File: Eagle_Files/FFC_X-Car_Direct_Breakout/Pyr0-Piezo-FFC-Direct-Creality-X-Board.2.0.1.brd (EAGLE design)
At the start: 48.1 x 50.7 mm, 11 parts, among them J1 FFC_MOLEX_0.5MM, J2 FFC_MOLEX_0.5MM

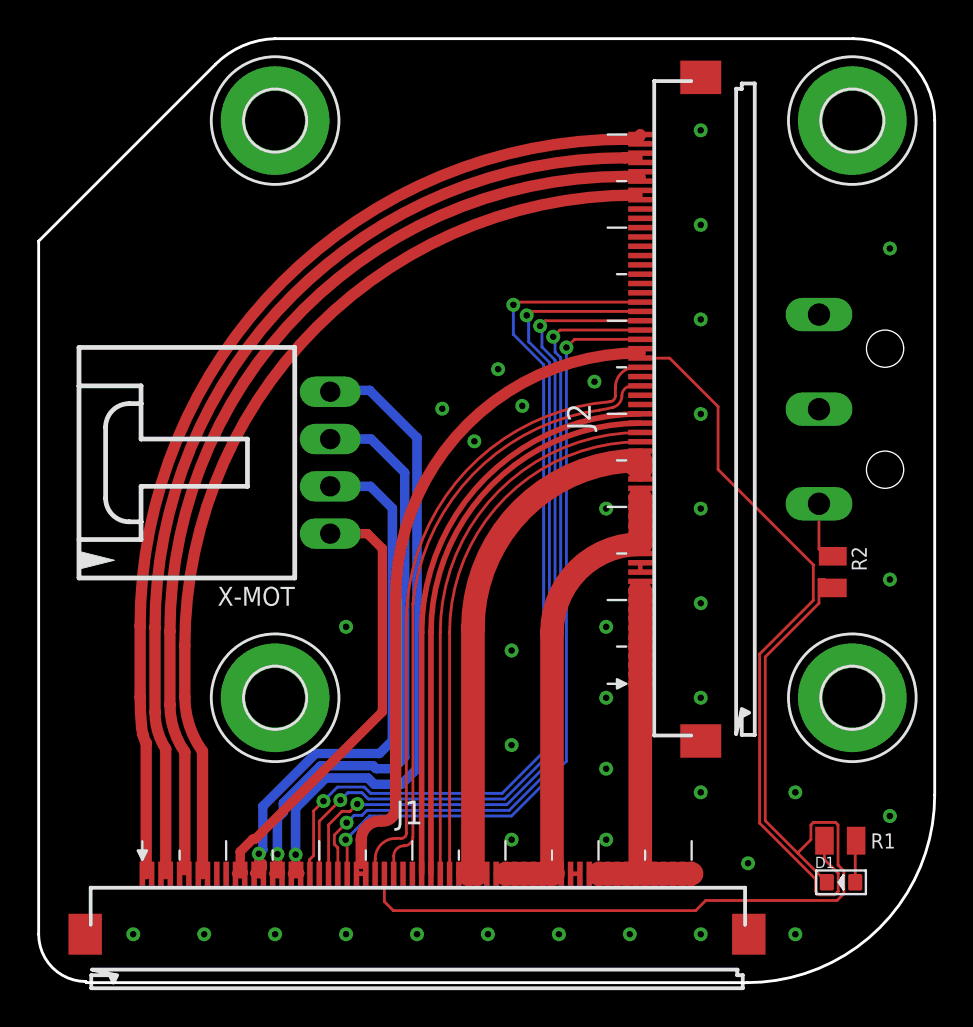
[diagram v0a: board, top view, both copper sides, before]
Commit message: Beta production board sync
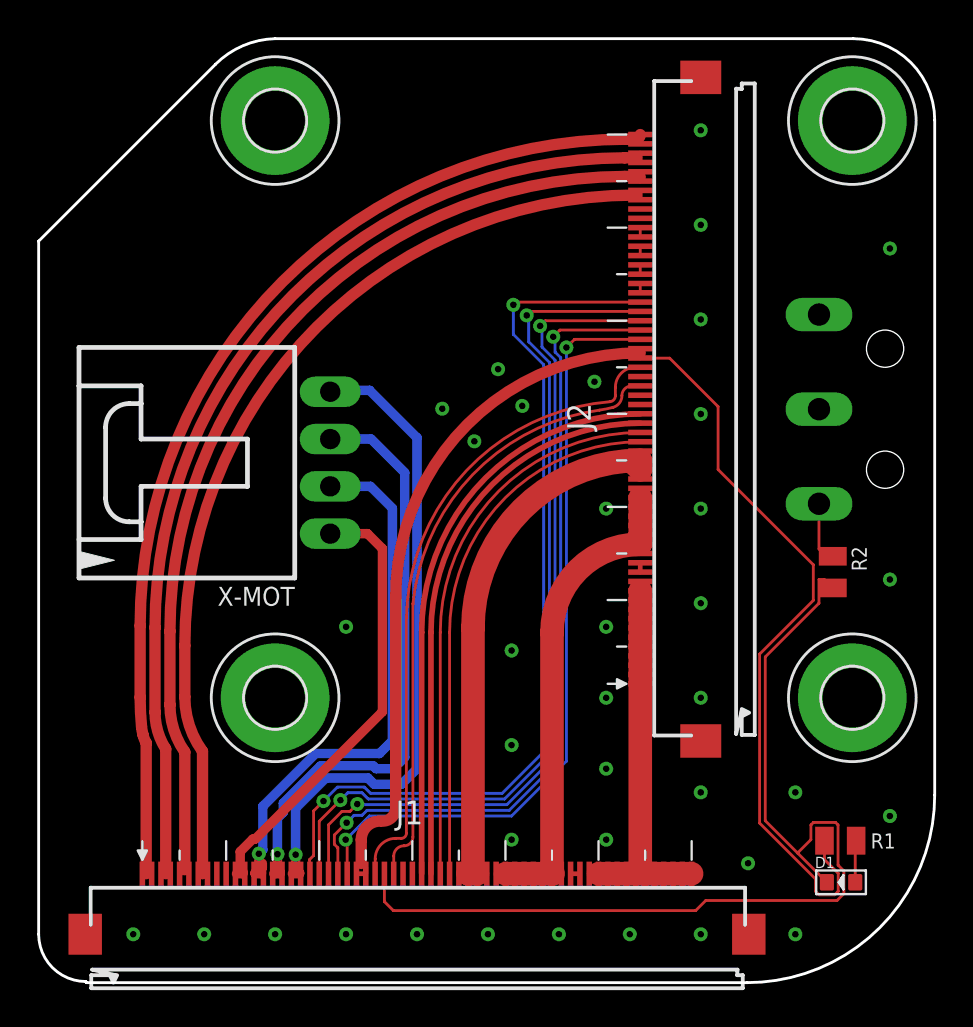
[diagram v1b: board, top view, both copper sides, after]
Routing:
- net X_2B: track 35.2 -> 35.7 mm
- net X_2B_NC: track 0.00 -> 0.50 mm
- net X_2A_NC: track 0.00 -> 0.50 mm
- net X_2A: track 32.0 -> 32.5 mm
- net X_1B_NC: track 0.00 -> 0.50 mm
- net X_1B: track 24.2 -> 24.7 mm
- net X_1A_NC: track 0.00 -> 0.50 mm
- net X_1A: track 29.4 -> 29.9 mm
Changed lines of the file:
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@@
 <drawing>
 <settings>
-<setting alwaysvectorfont="no"/>
+<setting alwaysvectorfont="yes"/>
 <setting verticaltext="up"/>
 </settings>
@@
 </layers>
 <board>
-<fusionsync huburn="a.cGVyc29uYWw6dWUyYTEyMDdh" projecturn="a.cGVyc29uYWw6dWUyYTEyMDdhIzIwMTgxMTI5MTYyOTY3NjMx" f3durn="urn:adsk.wipprod:dm.lineage:kuw35sM9Tt2kv8aK80rd8Q" pcbguid="e5e89037-45fa-459f-96bb-8df53076e544" lastpulledtime="" lastsyncedchangeguid="0a5c7ecb-5886-b503-4064-fa03a4f20b2b"/>
+<fusionsync huburn="a.cGVyc29uYWw6dWUyYTEyMDdh" projecturn="a.cGVyc29uYWw6dWUyYTEyMDdhIzIwMTgxMTI5MTYyOTY3NjMx" f3durn="urn:adsk.wipprod:dm.lineage:kuw35sM9Tt2kv8aK80rd8Q" pcbguid="e5e89037-45fa-459f-96bb-8df53076e544" lastpulledtime="" lastsyncedchangeguid="7aeb1a78-3c5e-2fd8-09c6-fdbde3539edf"/>
 <plain>
 <wire x1="-10.16" y1="-15.24" x2="-12.7" y2="-12.7" width="0.1524" layer="20" curve="-90"/>
@@
 <wire x1="-6.45" y1="3.775" x2="-6.45" y2="-0.775" width="0.6096" layer="1"/>
 <wire x1="-6.0228" y1="-9.45" x2="-5.875" y2="-9.45" width="0.1524" layer="1"/>
-<wire x1="-6.0228" y1="-9.45" x2="-6.13" y2="-9.45" width="0" layer="19" extent="1-1"/>
-<wire x1="-5.63" y1="-9.45" x2="-5.7372" y2="-9.45" width="0" layer="19" extent="1-1"/>
+<wire x1="-6.13" y1="-9.45" x2="-6.0228" y2="-9.45" width="0.1524" layer="1"/>
+<wire x1="-5.63" y1="-9.45" x2="-5.7372" y2="-9.45" width="0.1524" layer="1"/>
 </signal>
 <signal name="E0_2A">
@@
 <wire x1="-4.7372" y1="-9.3428" x2="-4.7372" y2="-9.45" width="0.1524" layer="1"/>
 <wire x1="-4.7372" y1="-9.45" x2="-5.0228" y2="-9.45" width="0.1524" layer="1"/>
-<wire x1="-5.0228" y1="-9.45" x2="-5.13" y2="-9.45" width="0" layer="19" extent="1-1"/>
-<wire x1="-4.63" y1="-9.45" x2="-4.7372" y2="-9.45" width="0" layer="19" extent="1-1"/>
+<wire x1="-5.0228" y1="-9.45" x2="-5.13" y2="-9.45" width="0.1524" layer="1"/>
+<wire x1="-4.63" y1="-9.45" x2="-4.7372" y2="-9.45" width="0.1524" layer="1"/>
 </signal>
 <signal name="E0_2B">
@@
 <contactref element="J2" pad="50"/>
 <contactref element="J2" pad="49"/>
-<wire x1="19.61" y1="24.75" x2="19.61" y2="25.25" width="0" layer="19" extent="1-1"/>
+<wire x1="19.61" y1="25.25" x2="19.61" y2="24.75" width="0.1524" layer="1"/>
 </signal>
 <signal name="X_1A_NC">
 <contactref element="J2" pad="48"/>
 <contactref element="J2" pad="47"/>
-<wire x1="19.61" y1="23.75" x2="19.61" y2="24.25" width="0" layer="19" extent="1-1"/>
+<wire x1="19.61" y1="24.25" x2="19.61" y2="23.75" width="0.1524" layer="1"/>
 </signal>
 <signal name="X_2A_NC">
 <contactref element="J2" pad="46"/>
 <contactref element="J2" pad="45"/>
-<wire x1="19.61" y1="22.75" x2="19.61" y2="23.25" width="0" layer="19" extent="1-1"/>
+<wire x1="19.61" y1="23.25" x2="19.61" y2="22.75" width="0.1524" layer="1"/>
 </signal>
 <signal name="X_2B_NC">
 <contactref element="J2" pad="44"/>
 <contactref element="J2" pad="43"/>
-<wire x1="19.61" y1="21.75" x2="19.61" y2="22.25" width="0" layer="19" extent="1-1"/>
+<wire x1="19.61" y1="22.25" x2="19.61" y2="21.75" width="0.1524" layer="1"/>
 </signal>
 <signal name="SDA">
@@
 <wire x1="-1.734" y1="-9.45" x2="-2.0736" y2="-9.45" width="0.508" layer="1"/>
 <wire x1="-1.875" y1="-8.26540625" x2="-1.875" y2="-9.205" width="0.508" layer="1"/>
-<wire x1="-2.0736" y1="-9.45" x2="-2.13" y2="-9.45" width="0" layer="19" extent="1-1"/>
-<wire x1="-1.63" y1="-9.45" x2="-1.734" y2="-9.45" width="0" layer="19" extent="1-1"/>
+<wire x1="-1.734" y1="-9.45" x2="-1.63" y2="-9.45" width="0.1524" layer="1"/>
+<wire x1="-2.13" y1="-9.45" x2="-1.734" y2="-9.45" width="0.1524" layer="1"/>
 </signal>
 <signal name="X_1A">
@@
 <wire x1="-0.6864" y1="-9.12885" x2="-0.6864" y2="-8.89" width="0.508" layer="1"/>
 <wire x1="6.2992" y1="10.1758" x2="6.2992" y2="-2.3008" width="0.508" layer="16"/>
-<wire x1="-1.0736" y1="-9.45" x2="-1.13" y2="-9.45" width="0" layer="19" extent="1-1"/>
-<wire x1="-0.63" y1="-9.45" x2="-0.734" y2="-9.45" width="0" layer="19" extent="1-1"/>
+<wire x1="-0.734" y1="-9.45" x2="-0.63" y2="-9.45" width="0.1524" layer="1"/>
+<wire x1="-1.13" y1="-9.45" x2="-0.734" y2="-9.45" width="0.1524" layer="1"/>
 </signal>
 <signal name="X_2A">
@@
 <wire x1="0.125" y1="-9.205" x2="0.266" y2="-9.346" width="0.508" layer="1"/>
 <wire x1="0.266" y1="-9.346" x2="0.266" y2="-9.45" width="0.508" layer="1"/>
-<wire x1="0.266" y1="-9.45" x2="-0.0736" y2="-9.45" width="0.508" layer="1"/>
+<wire x1="0.266" y1="-9.45" x2="0" y2="-9.45" width="0.508" layer="1"/>
+<wire x1="0" y1="-9.45" x2="-0.0736" y2="-9.45" width="0.508" layer="1"/>
 <wire x1="6.9596" y1="12.0904" x2="6.9596" y2="-3.2004" width="0.508" layer="16"/>
-<wire x1="-0.0736" y1="-9.45" x2="-0.13" y2="-9.45" width="0" layer="19" extent="1-1"/>
-<wire x1="0.37" y1="-9.45" x2="0.266" y2="-9.45" width="0" layer="19" extent="1-1"/>
+<wire x1="0" y1="-9.45" x2="0.37" y2="-9.45" width="0.1524" layer="1"/>
+<wire x1="-0.13" y1="-9.45" x2="0" y2="-9.45" width="0.1524" layer="1"/>
 </signal>
 <signal name="X_2B">
@@
 <wire x1="1.3136" y1="-9.3936" x2="1.3136" y2="-9.45" width="0.508" layer="1"/>
 <wire x1="1.3136" y1="-9.45" x2="0.9264" y2="-9.45" width="0.508" layer="1"/>
-<wire x1="0.9264" y1="-9.45" x2="0.87" y2="-9.45" width="0" layer="19" extent="1-1"/>
-<wire x1="1.37" y1="-9.45" x2="1.3136" y2="-9.45" width="0" layer="19" extent="1-1"/>
+<wire x1="0.87" y1="-9.45" x2="1.3136" y2="-9.45" width="0.1524" layer="1"/>
+<wire x1="1.37" y1="-9.45" x2="1.3136" y2="-9.45" width="0.1524" layer="1"/>
 </signal>
 <signal name="Z_MIN_TRIG">
